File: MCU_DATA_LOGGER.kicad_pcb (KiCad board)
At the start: 2 copper layers, 49.3 x 31.2 mm, 29 parts, among them J1 Conn_01x04_Male, J2 Conn_01x04_Male, J3 Conn_01x09_Male, J4 Conn_02x03_Odd_Even, U1 DS1337S+, U2 24LC1025, U3 24LC1025, U4 ATMEGA328P-AU, Y1 32.768 KHz, Y2 16 MHz

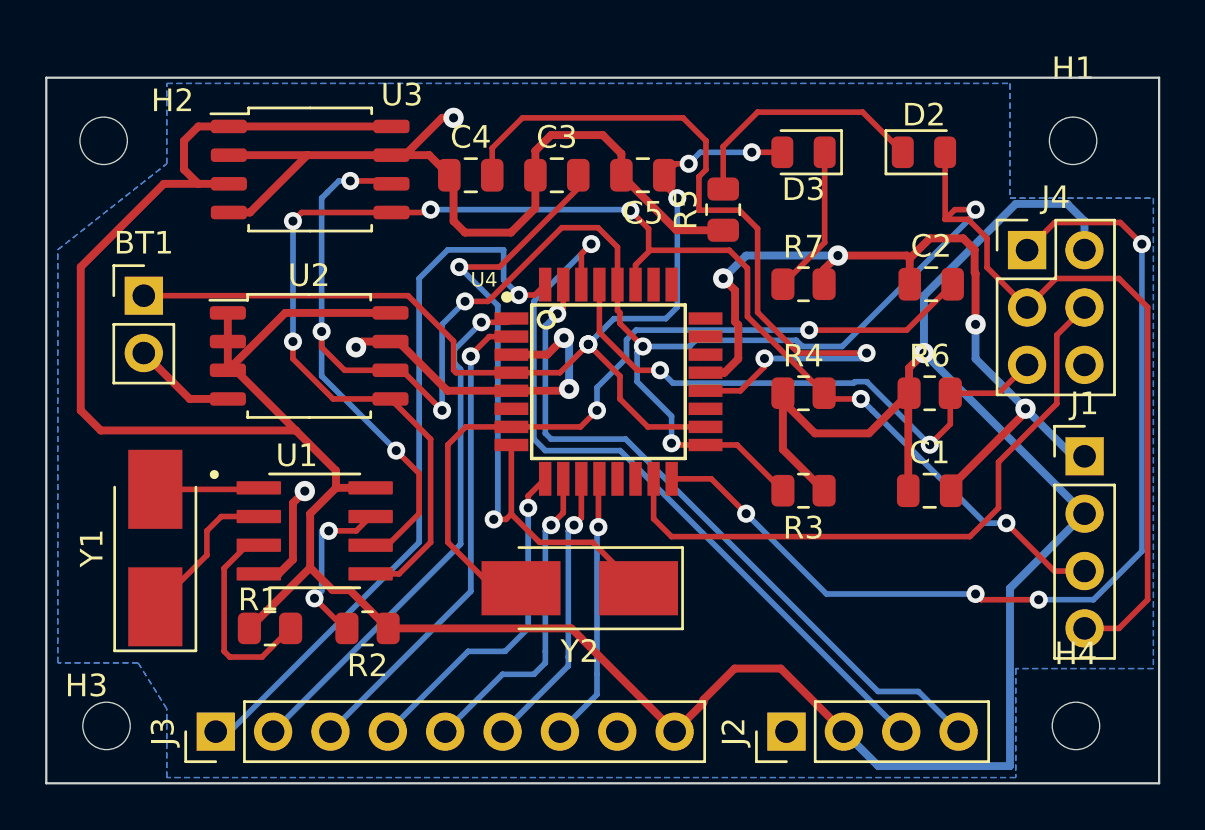
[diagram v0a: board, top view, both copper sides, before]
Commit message: fixed all issues
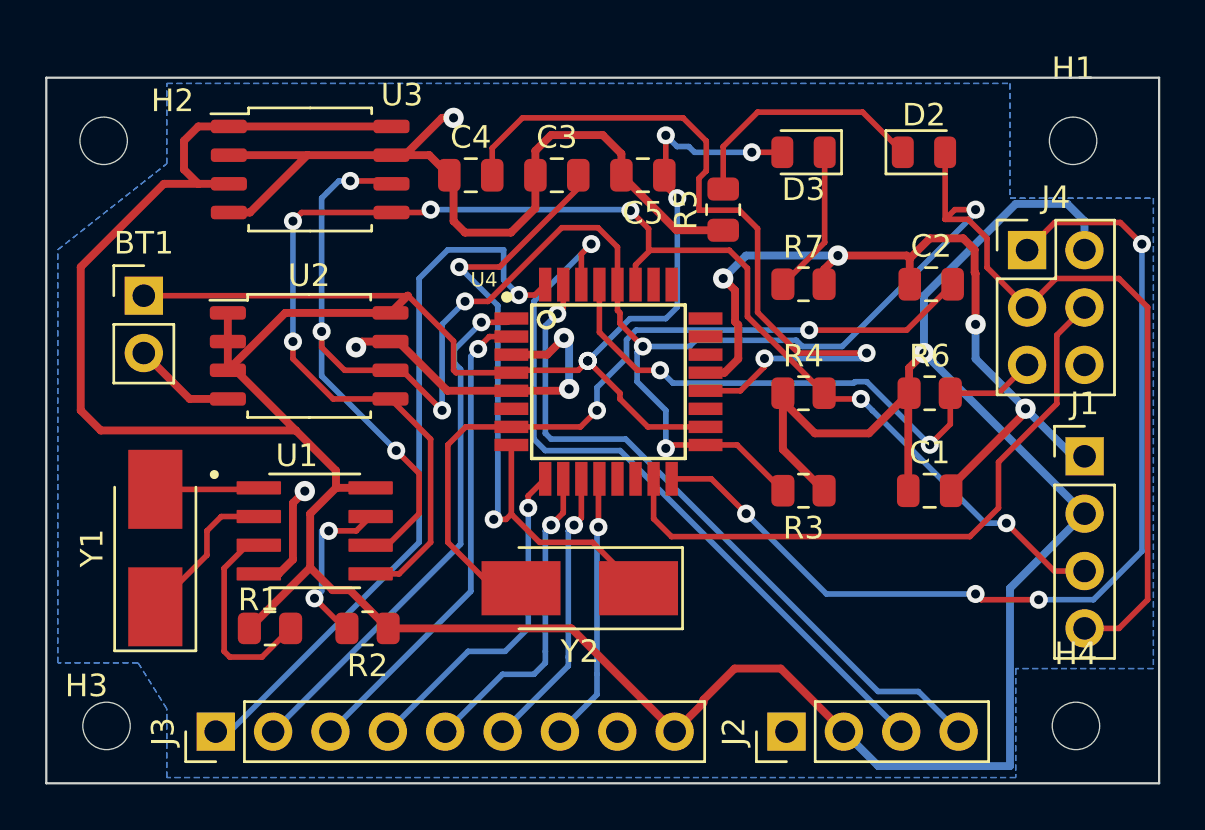
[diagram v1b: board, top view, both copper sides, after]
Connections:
- BT1 pad 1: Net-(BT1-Pad1) -> /Vcc
- C5 pad 1: Net-(BT1-Pad1) -> /Vcc
- D3 pad 2: Net-(BT1-Pad1) -> /Vcc
- U4 pad 18: Net-(BT1-Pad1) -> /Vcc
- U4 pad 4: Net-(BT1-Pad1) -> /Vcc
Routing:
- net /Vcc: track 154.9 -> 203.0 mm, vias 1 -> 6
- net Net-(BT1-Pad1): track 46.0 -> 0.00 mm, vias 5 -> 0
